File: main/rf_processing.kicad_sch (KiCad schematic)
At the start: 13 parts

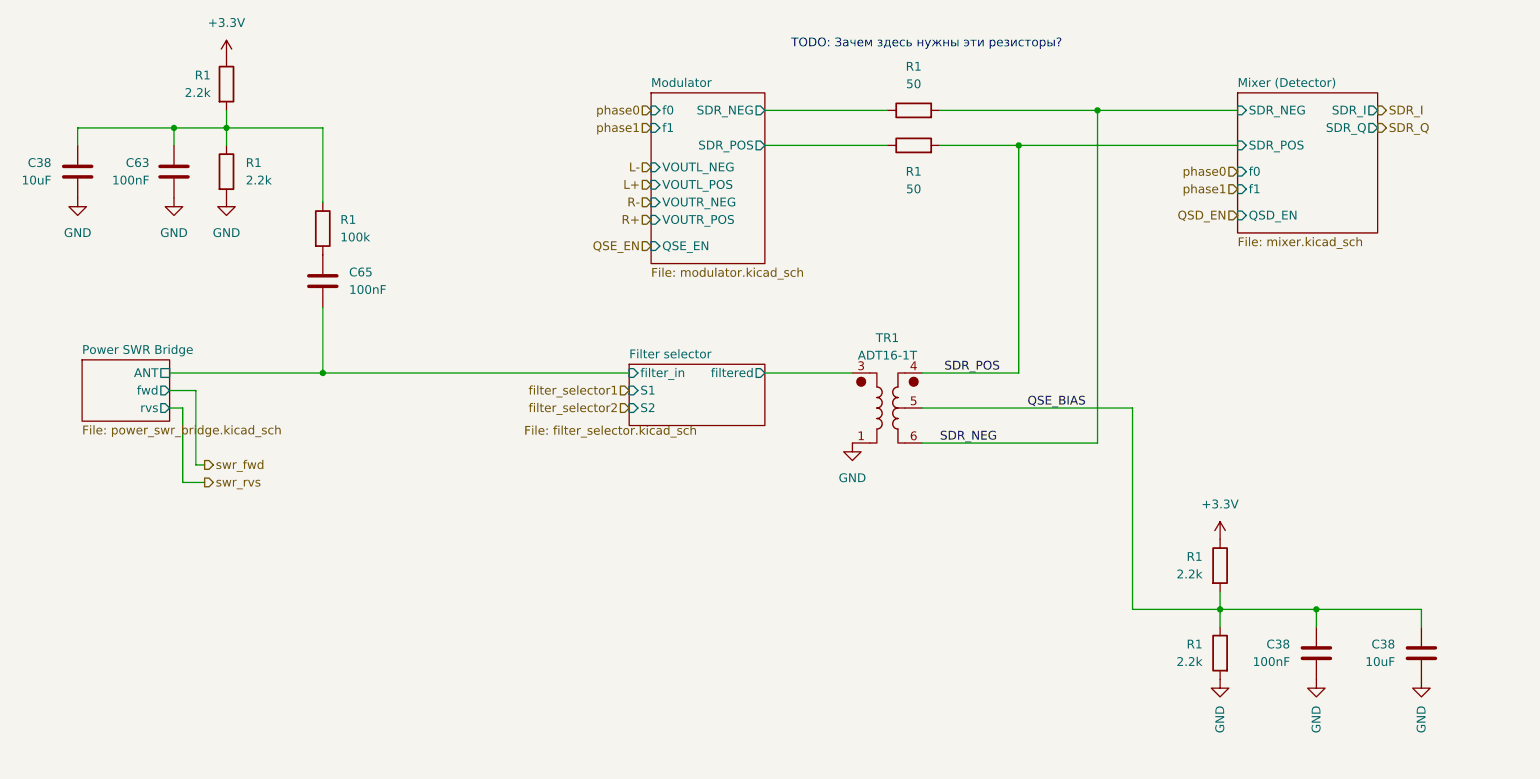
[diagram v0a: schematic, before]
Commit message: Amplifier added to circuit
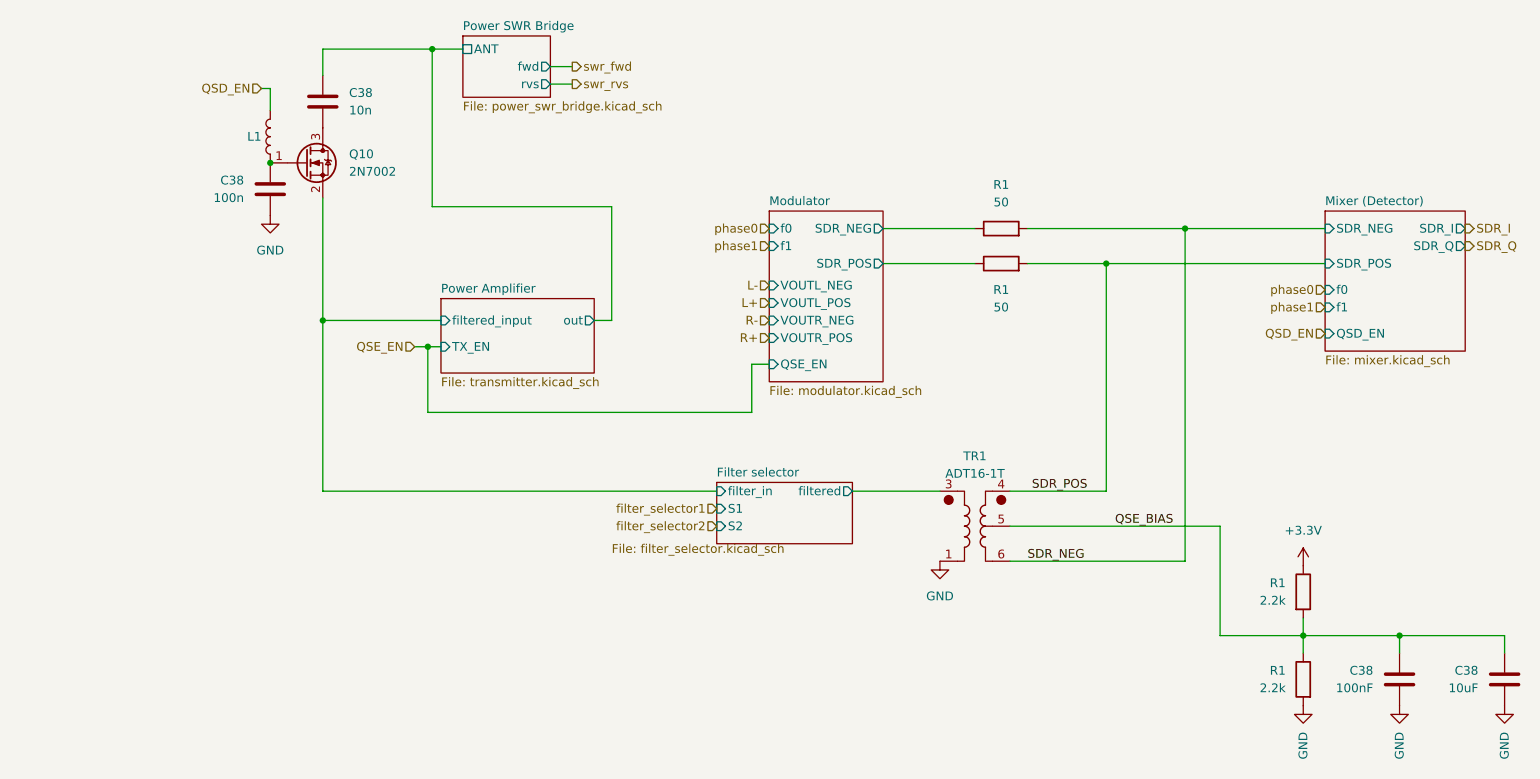
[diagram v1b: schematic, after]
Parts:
- removed C38: 10uF, symbol Device:C
- removed C63, C65: 100nF, symbol Device:C
- removed R1: 100k, symbol Device:R
- removed R1 (x2): 2.2k, symbol Device:R
- added C38: 100n, symbol Device:C
- added C38: 10n, symbol Device:C
- added L1: ~, symbol Device:L
- added Q10: 2N7002, Package_TO_SOT_SMD:SOT-23, symbol Transistor_FET:2N7002
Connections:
- net Filter selector/filter_in: now also Q10.2 (S)
- net GND: now also C38.1
- net QSD_EN: now also L1.1
- new net: C38.2, L1.2, Q10.1 (G)
- new net: C38.1, Q10.3 (D)
- new net Power Amplifier/out: C38.2
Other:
- added sheet Power Amplifier (transmitter.kicad_sch)
- note removed: "TODO: Зачем здесь нужны эти резисторы?"
- moved on the sheet: C38, R1, TR1
